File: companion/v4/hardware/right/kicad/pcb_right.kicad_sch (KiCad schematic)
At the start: 27 parts, among them J1 TF31-6S-0.5SH_800_, J2 speaker, J3 USB_C_Receptacle_USB2.0_14P, SW1 SW_Push, SW2 SW_Push, U1 AP2112K-3.3, U2 MAX98357AETE_T, U3 ESP32-C6-MINI-1

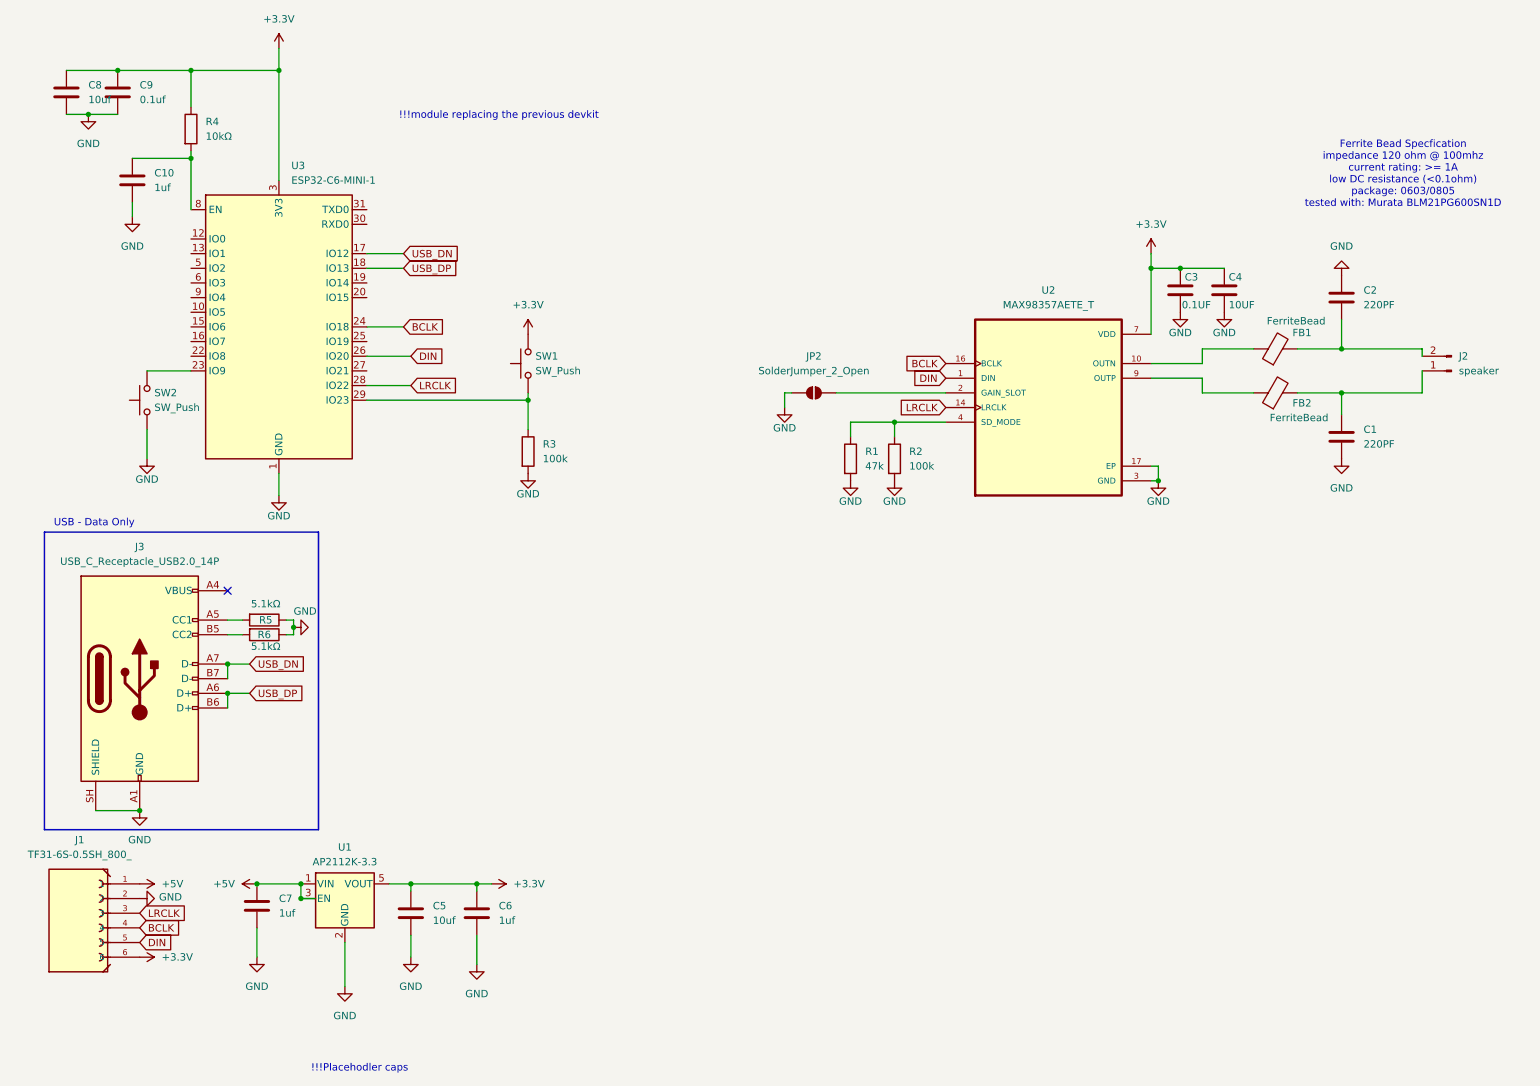
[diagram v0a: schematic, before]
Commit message: fixes
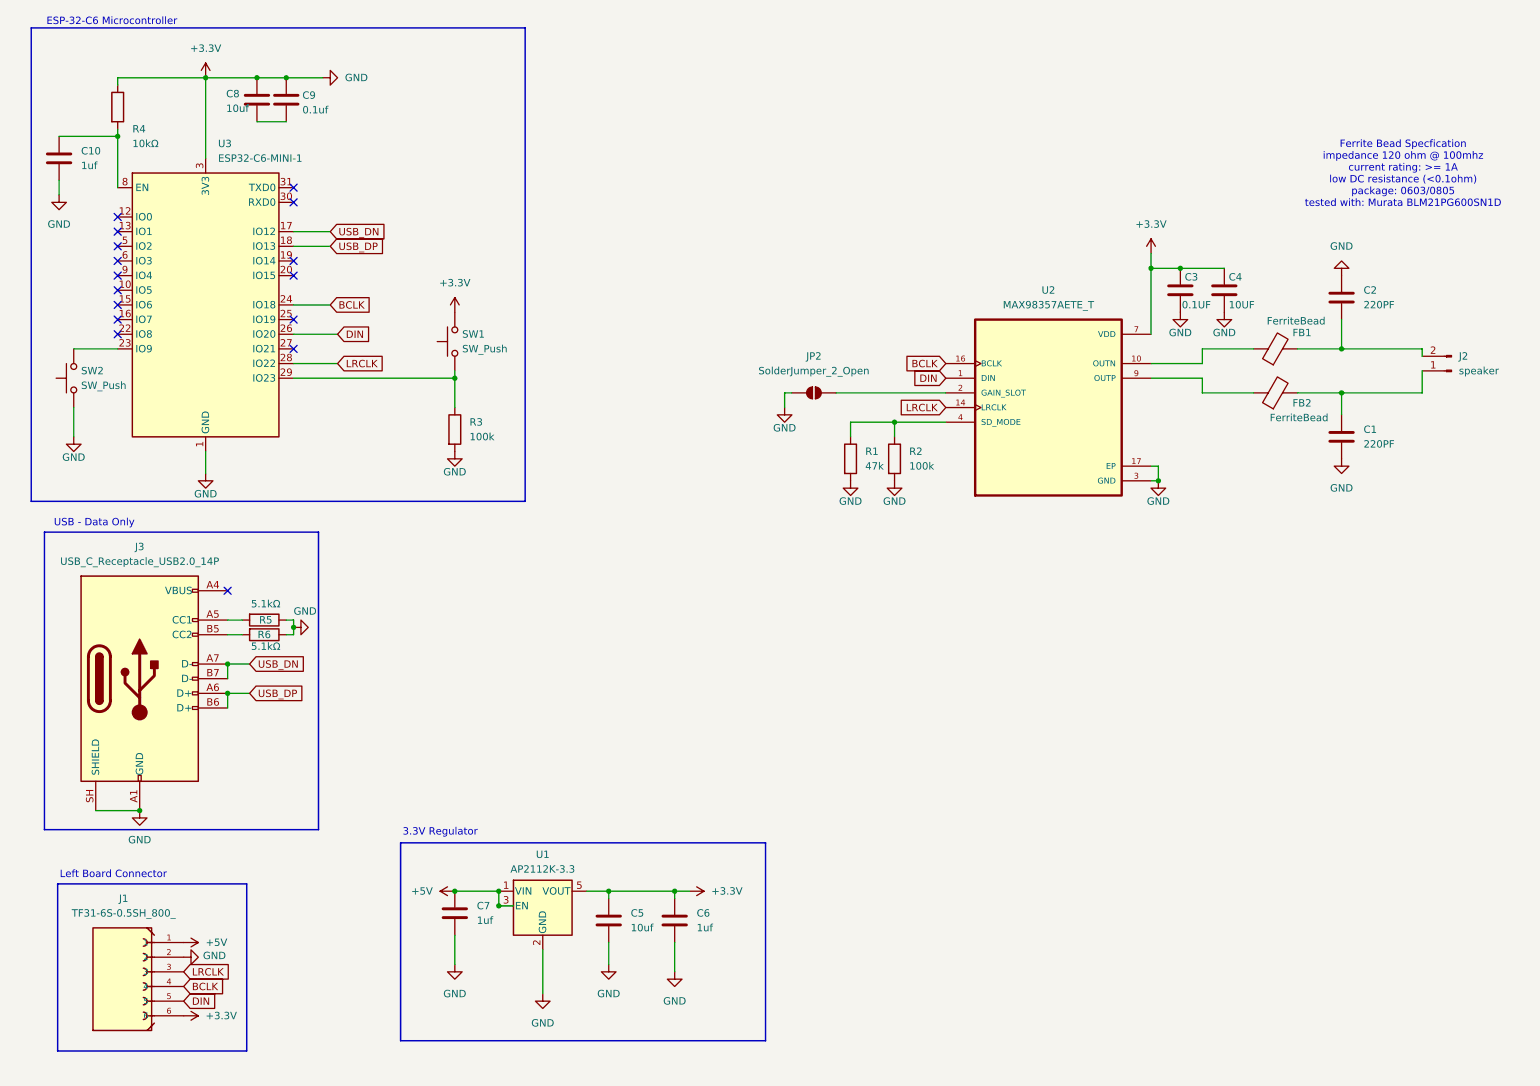
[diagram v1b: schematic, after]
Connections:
- net +3.3V: now also C1.2, C10.2, C2.1, C3.2, C4.2, C5.2, C6.2, C7.2, J1.2, J3.A1 (GND), J3.A12 (GND), J3.B1 (GND), J3.B12 (GND), J3.SH (SHIELD), JP2.1 (A), R1.2, R2.2, R3.2, R5.1, R6.1, SW2.1, U1.2 (GND), U2.11 (GND), U2.15 (GND), U2.17 (EP), U2.3 (GND), U3.1 (GND), U3.11 (GND), U3.14 (GND), U3.2 (GND), U3.36 (GND), U3.37 (GND), U3.38 (GND), U3.39 (GND), U3.40 (GND), U3.41 (GND), U3.42 (GND), U3.43 (GND), U3.44 (GND), U3.45 (GND), U3.46 (GND), U3.47 (GND), U3.48 (GND), U3.49 (GND), U3.50 (GND), U3.51 (GND), U3.52 (GND), U3.53 (GND)
- removed net GND: C1.2, C10.2, C2.1, C3.2, C4.2, C5.2, C6.2, C7.2, C8.2, C9.2, J1.2, J3.A1 (GND), J3.A12 (GND), J3.B1 (GND), J3.B12 (GND), J3.SH (SHIELD), JP2.1 (A), R1.2, R2.2, R3.2, R5.1, R6.1, SW2.1, U1.2 (GND), U2.11 (GND), U2.15 (GND), U2.17 (EP), U2.3 (GND), U3.1 (GND), U3.11 (GND), U3.14 (GND), U3.2 (GND), U3.36 (GND), U3.37 (GND), U3.38 (GND), U3.39 (GND), U3.40 (GND), U3.41 (GND), U3.42 (GND), U3.43 (GND), U3.44 (GND), U3.45 (GND), U3.46 (GND), U3.47 (GND), U3.48 (GND), U3.49 (GND), U3.50 (GND), U3.51 (GND), U3.52 (GND), U3.53 (GND)
- new net: C8.2, C9.2
- no-connect marks 1 -> 16
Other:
- note added: "3.3V Regulator"
- note added: "ESP-32-C6 Microcontroller"
- note added: "Left Board Connector"
- note removed: "!!!Placehodler caps"
- note removed: "!!!module replacing the previous devkit"
- moved on the sheet: C10, C5, C6, C7, C8, C9, J1, R3, R4, SW1, SW2, U1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
